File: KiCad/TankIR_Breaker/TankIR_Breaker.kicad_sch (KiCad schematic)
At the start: 17 parts, among them J1 VBATT, J2 TRIGGER, J3 SERVO, J4 RC, J5 APPLE, J6 SOUND, J7 IR_OUT, J8 MUZZLE, Q1 BC337, Q2 BC337, U1 LM7805_TO220

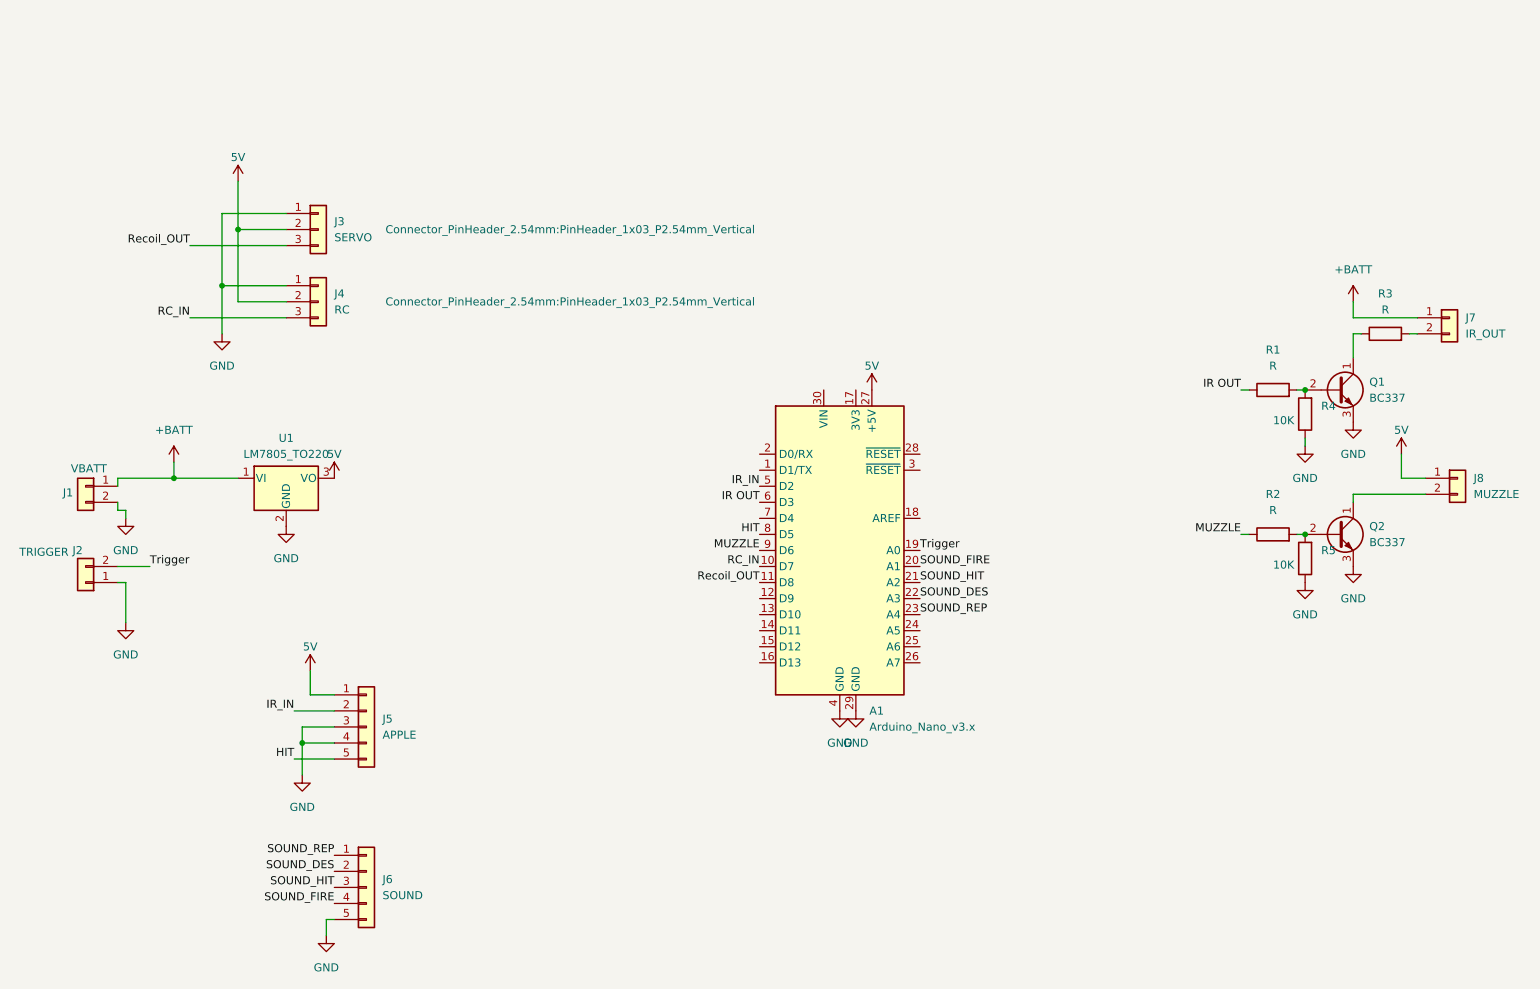
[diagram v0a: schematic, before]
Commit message: Correction
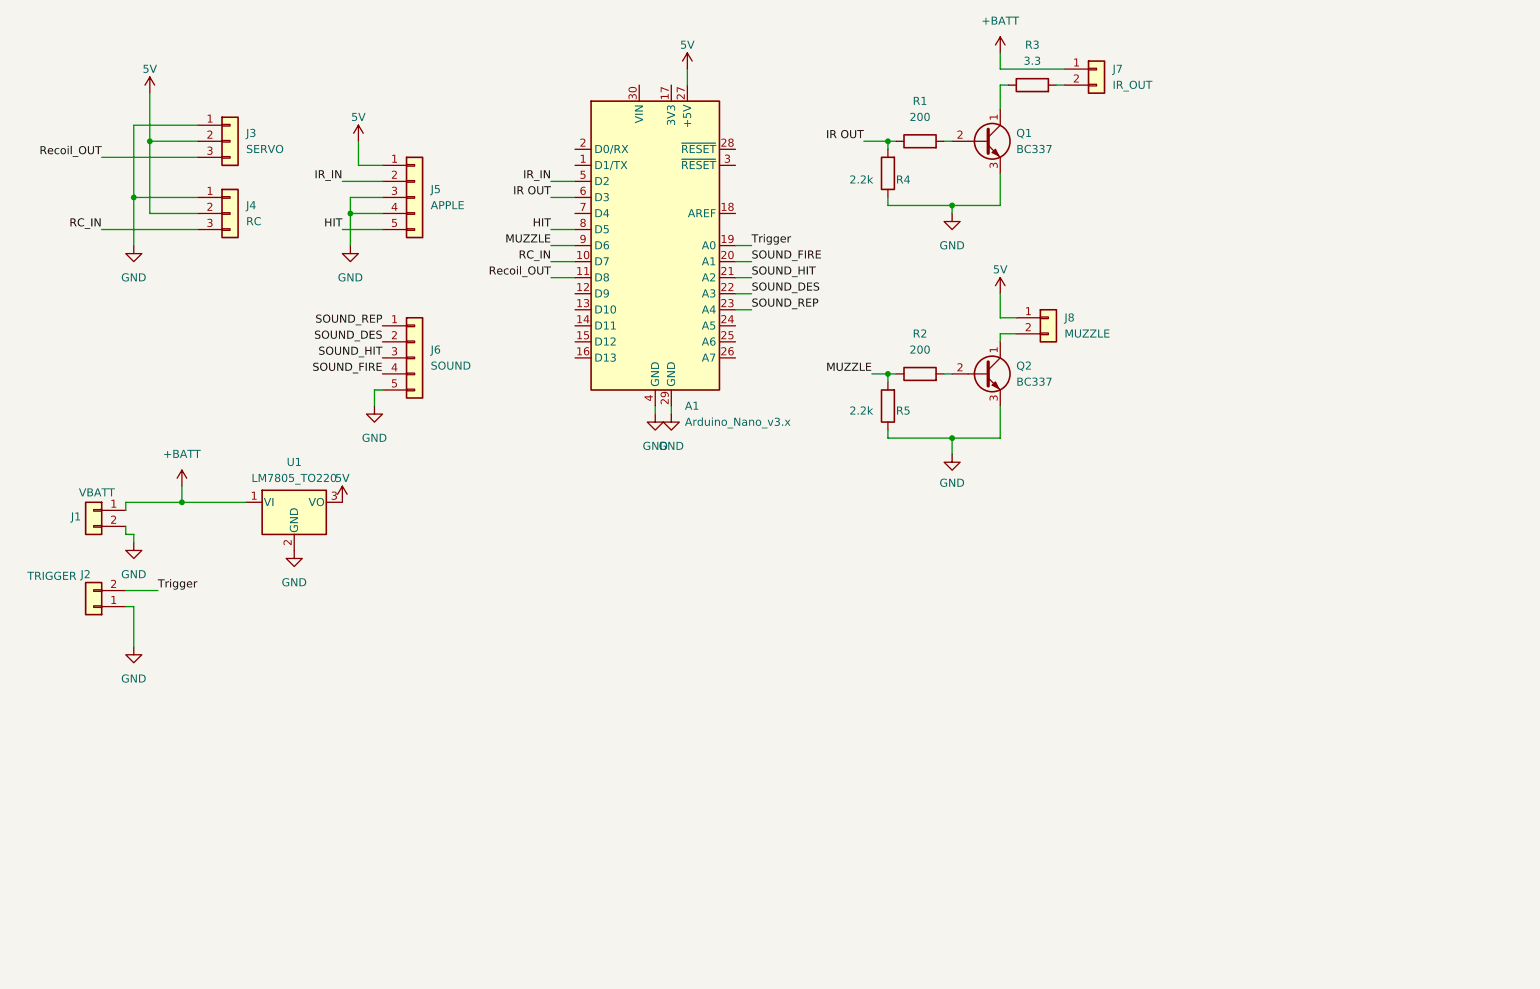
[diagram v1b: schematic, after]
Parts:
- R1, R2: value R -> 200
- R3: value R -> 3.3
- R4, R5: value 10K -> 2.2k
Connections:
- net IR OUT: now also R4.2
- net MUZZLE: now also R5.2
- net at Q1.2 (B), R1.2: no longer R4.2
- net at Q2.2 (B), R2.2: no longer R5.2
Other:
- moved on the sheet: A1, J1, J2, J3, J4, J5, J6, J7, J8, Q1, Q2, R1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
